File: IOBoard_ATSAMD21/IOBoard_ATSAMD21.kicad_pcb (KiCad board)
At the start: 2 copper layers, 76.2 x 128.5 mm, 36 parts, among them J1 Conn_PIC_ICSP_ICD, J2 Conn_01x04_Male, SW1 EG_1218, SW2 EG_1218, SW3 EG_1218, SW4 EG_1218, U1 ATSAMD21G18A-A, U2 AP2112K-3.3

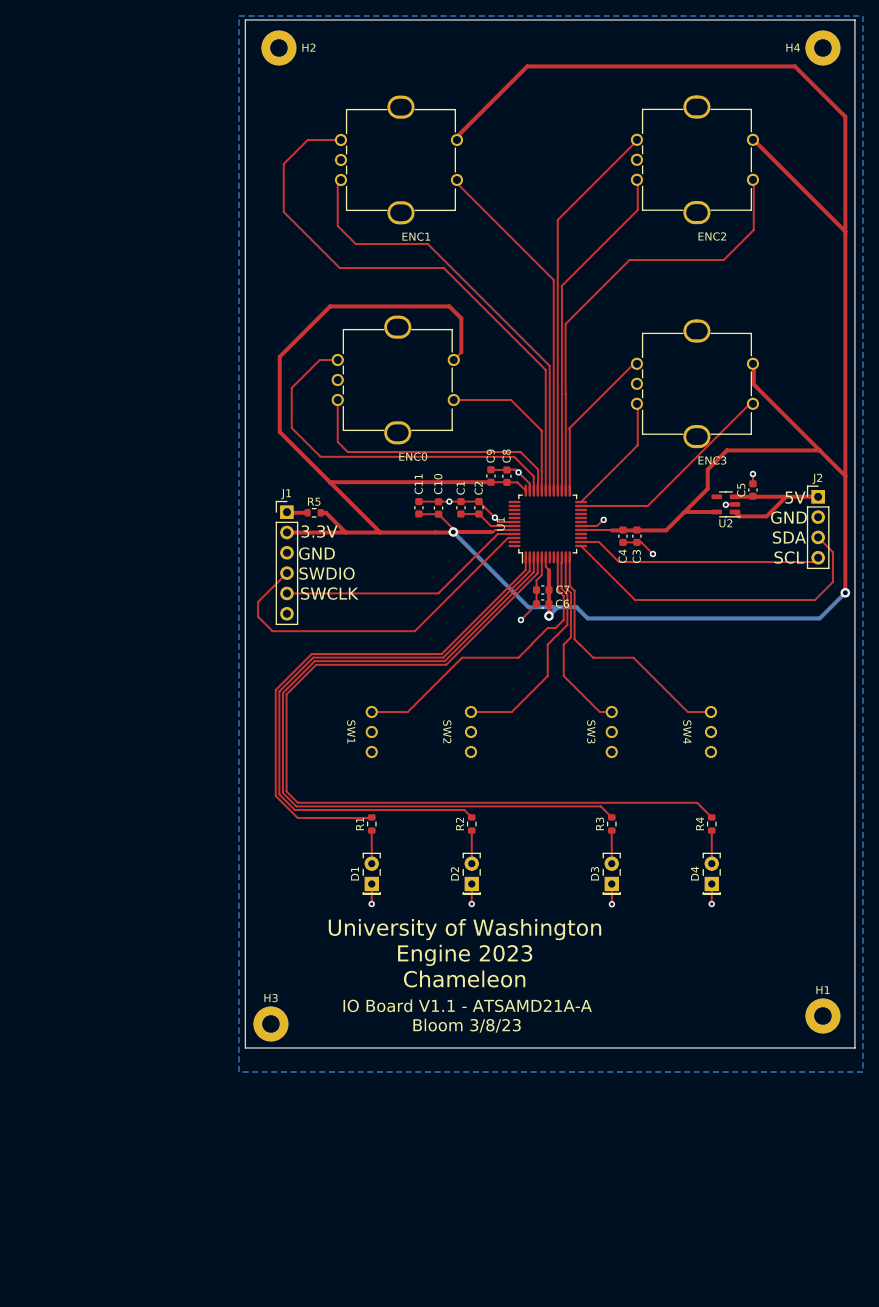
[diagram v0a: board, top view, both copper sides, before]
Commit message: IOBoard V2 + documentation
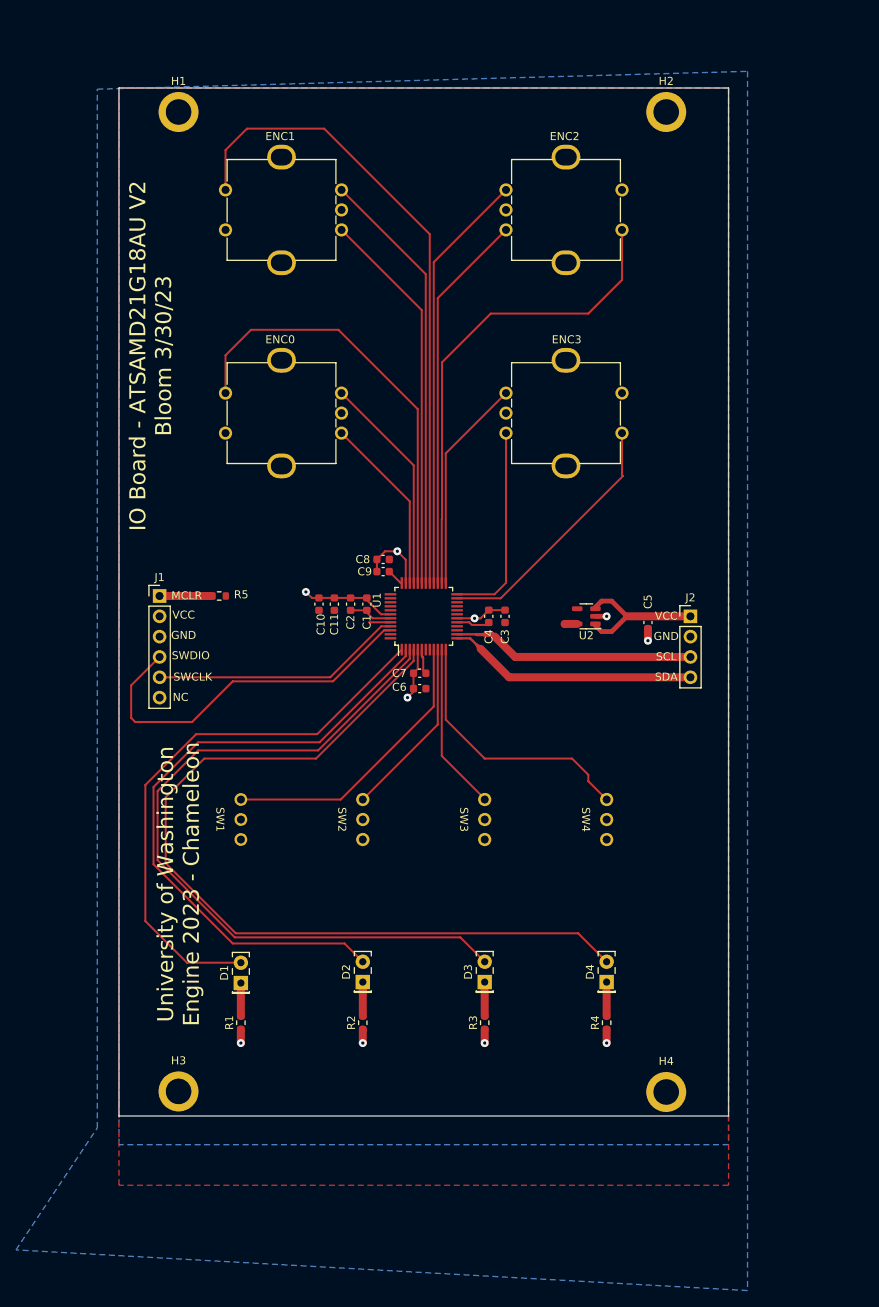
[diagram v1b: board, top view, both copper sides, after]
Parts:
- H1, H2, H3, H4: footprint MountingHole:MountingHole_2.2mm_M2_Pad -> MountingHole:MountingHole_3.2mm_M3_ISO7380_Pad
- SW1, SW2, SW3, SW4: footprint Custom:EG_1218 -> custom_lib:EG_1218
- moved H1 138.8 mm to (57.5, 53.0)
- moved H4 132.0 mm to (118.4, 175.5)
- moved H2 49.1 mm to (118.4, 53.0)
- moved R1 29.7 mm to (65.2, 166.8)
- moved R3 29.5 mm to (95.7, 166.8)
- moved R2 28.3 mm to (80.5, 166.8)
- moved R4 28.1 mm to (111.0, 166.8)
- moved SW3 23.6 mm to (95.7, 141.4)
- moved U2 22.4 mm to (108.4, 116.0)
- moved J2 21.9 mm to (121.4, 116.0)
- moved SW2 21.5 mm to (80.5, 141.4)
- moved C5 21.1 mm to (116.1, 116.8), turned to -90 degrees
- moved SW4 21.1 mm to (111.0, 141.4)
- moved D1 20.5 mm to (65.2, 161.9)
- moved D3 20.1 mm to (95.7, 161.8)
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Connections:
- D1 pad 1: GND -> Net-(D1-Pad1)
- D1 pad 2: Net-(D1-Pad2) -> /LED0
- D2 pad 1: GND -> Net-(D2-Pad1)
- D2 pad 2: Net-(D2-Pad2) -> /LED1
- D3 pad 1: GND -> Net-(D3-Pad1)
- D3 pad 2: Net-(D3-Pad2) -> /LED2
- D4 pad 1: GND -> Net-(D4-Pad1)
- D4 pad 2: Net-(D4-Pad2) -> /LED3
- J2 pad 3: /SDA -> /SCL
- J2 pad 4: /SCL -> /SDA
- R1 pad 1: Net-(D1-Pad2) -> GND
- R1 pad 2: /LED0 -> Net-(D1-Pad1)
- R2 pad 1: Net-(D2-Pad2) -> GND
- R2 pad 2: /LED1 -> Net-(D2-Pad1)
- R3 pad 1: Net-(D3-Pad2) -> GND
- R3 pad 2: /LED2 -> Net-(D3-Pad1)
- R4 pad 1: Net-(D4-Pad2) -> GND
- R4 pad 2: /LED3 -> Net-(D4-Pad1)
- SW1 pad 1: GND -> +3.3V
- SW2 pad 1: GND -> +3.3V
- SW3 pad 1: GND -> +3.3V
- SW4 pad 1: GND -> +3.3V
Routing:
- net +3.3V: track 375.8 -> 13.9 mm, vias 3 -> 0
- net /ENC1_SW: track 44.0 -> 80.7 mm
- net /ENC0_SW: track 21.4 -> 55.9 mm
- net /ENC0_A: track 46.7 -> 22.3 mm
- net /ENC1_A: track 70.0 -> 48.3 mm
- net /SDA: track 41.6 -> 31.2 mm
- net /ENC3_B: track 15.7 -> 25.4 mm
- net /ENC0_B: track 34.5 -> 27.5 mm
- net /ENC3_A: track 19.9 -> 26.9 mm
- net /ENC3_SW: track 27.1 -> 32.5 mm
- net GND: track 48.4 -> 43.2 mm, vias 12 -> 10
- net /ENC2_SW: track 55.5 -> 60.6 mm
- net /ENC2_B: track 42.8 -> 47.7 mm
- net /ENC2_A: track 48.0 -> 52.9 mm
- net /LED0: track 65.5 -> 70.2 mm
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- added copper zone on F.Cu, net +3.3V
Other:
- board text added: "IO Board - ATSAMD21G18AU V2 Bloom 3/30/23"
- board text added: "MCLR"
- board text added: "NC"
- board text added: "University of Washington Engine 2023 - Chameleon"
- board text added: "VCC"
- board text removed: "3.3V"
- board text removed: "5V"
- board text removed: "IO Board V1.1 - ATSAMD21A-A Bloom 3/8/23"
- board text removed: "IOBoard ATSAMD21 V1"
- board text removed: "University of Washington Engine 2023 Chameleon"
